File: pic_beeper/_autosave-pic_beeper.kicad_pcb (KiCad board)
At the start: 2 copper layers, 33 x 26.7 mm, 7 parts, among them J1 Conn_01x06, SW1 SW_SPDT, U1 PIC12F752-IP

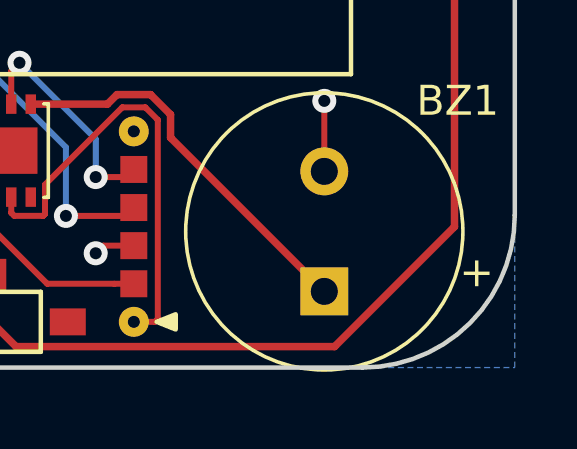
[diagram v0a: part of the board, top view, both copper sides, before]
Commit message: Finish v1.0
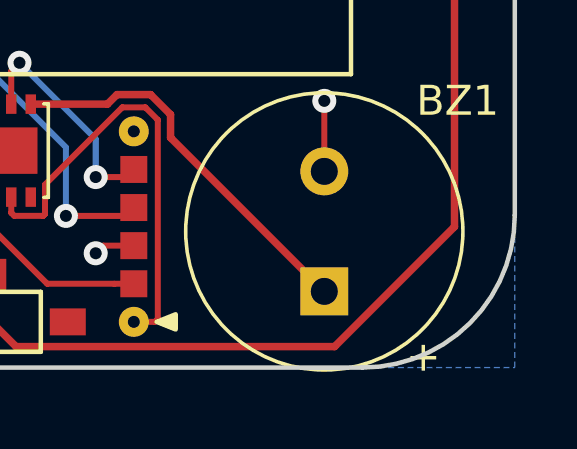
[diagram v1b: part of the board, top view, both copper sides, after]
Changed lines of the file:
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@@
       (outputformat 1)
       (mirror false)
-      (drillshape 1)
+      (drillshape 0)
       (scaleselection 1)
-      (outputdirectory ""))
+      (outputdirectory "plots/"))
   )
   (net 0 "")
@@
       (effects (font (size 1 1) (thickness 0.15)))
     )
-    (fp_text user + (at -5.08 0.635 180) (layer F.SilkS)
+    (fp_text user + (at -3.3 -2.18 180) (layer F.SilkS)
       (effects (font (size 1 1) (thickness 0.15)))
     )
@@
     (pad 6 thru_hole circle (at 2.794 0 90) (size 1 1) (drill 0.4) (layers *.Cu *.Mask)
       (net 8 "Net-(J1-Pad6)"))
-    (pad 5 smd rect (at 1.524 0 90) (size 0.9 0.9) (layers F.Cu F.Paste F.Mask)
+    (pad 5 smd rect (at 1.524 0 90) (size 0.9 0.9) (layers F.Cu F.Mask)
       (net 7 /ICSPCLK))
-    (pad 4 smd rect (at 0.254 0 90) (size 0.9 0.9) (layers F.Cu F.Paste F.Mask)
+    (pad 4 smd rect (at 0.254 0 90) (size 0.9 0.9) (layers F.Cu F.Mask)
       (net 6 /ICSPDAT))
-    (pad 3 smd rect (at -1.016 0 90) (size 0.9 0.9) (layers F.Cu F.Paste F.Mask)
-      (net 2 -BATT))
-    (pad 2 smd rect (at -2.286 0 90) (size 0.9 0.9) (layers F.Cu F.Paste F.Mask)
+    (pad 3 smd rect (at -1.016 0 90) (size 0.9 0.9) (layers F.Cu F.Mask)
+      (net 2 -BATT))
+    (pad 2 smd rect (at -2.286 0 90) (size 0.9 0.9) (layers F.Cu F.Mask)
       (net 4 +BATT))
     (pad 1 thru_hole circle (at -3.556 0 90) (size 1 1) (drill 0.4) (layers *.Cu *.Mask)
@@
       (effects (font (size 1 1) (thickness 0.15)))
     )
+    (fp_circle (center 0 0) (end 3.75 0) (layer F.CrtYd) (width 0.05))
+    (fp_circle (center 0 0) (end 3.5 0) (layer Cmts.User) (width 0.15))
     (fp_text user %R (at 0.3 0) (layer F.Fab)
       (effects (font (size 1 1) (thickness 0.15)))
     )
-    (fp_circle (center 0 0) (end 3.5 0) (layer Cmts.User) (width 0.15))
-    (fp_circle (center 0 0) (end 3.75 0) (layer F.CrtYd) (width 0.05))
+    (pad 1 thru_hole circle (at 1.856155 -1.856155) (size 0.8 0.8) (drill 0.5) (layers *.Cu *.Mask)
+      (net 2 -BATT))
+    (pad 1 thru_hole circle (at 0 -2.625) (size 0.8 0.8) (drill 0.5) (layers *.Cu *.Mask)
+      (net 2 -BATT))
+    (pad 1 thru_hole circle (at -1.856155 -1.856155) (size 0.8 0.8) (drill 0.5) (layers *.Cu *.Mask)
+      (net 2 -BATT))
+    (pad 1 thru_hole circle (at -2.625 0) (size 0.8 0.8) (drill 0.5) (layers *.Cu *.Mask)
+      (net 2 -BATT))
+    (pad 1 thru_hole circle (at -1.856155 1.856155) (size 0.8 0.8) (drill 0.5) (layers *.Cu *.Mask)
+      (net 2 -BATT))
+    (pad 1 thru_hole circle (at 0 2.625) (size 0.8 0.8) (drill 0.5) (layers *.Cu *.Mask)
+      (net 2 -BATT))
+    (pad 1 thru_hole circle (at 1.856155 1.856155) (size 0.8 0.8) (drill 0.5) (layers *.Cu *.Mask)
+      (net 2 -BATT))
+    (pad 1 thru_hole circle (at 2.625 0) (size 0.8 0.8) (drill 0.5) (layers *.Cu *.Mask)
+      (net 2 -BATT))
     (pad 1 thru_hole circle (at 0 0) (size 7 7) (drill 3.5) (layers *.Cu *.Mask)
       (net 2 -BATT))
-    (pad 1 thru_hole circle (at 2.625 0) (size 0.8 0.8) (drill 0.5) (layers *.Cu *.Mask)
-      (net 2 -BATT))
-    (pad 1 thru_hole circle (at 1.856155 1.856155) (size 0.8 0.8) (drill 0.5) (layers *.Cu *.Mask)
-      (net 2 -BATT))
-    (pad 1 thru_hole circle (at 0 2.625) (size 0.8 0.8) (drill 0.5) (layers *.Cu *.Mask)
-      (net 2 -BATT))
-    (pad 1 thru_hole circle (at -1.856155 1.856155) (size 0.8 0.8) (drill 0.5) (layers *.Cu *.Mask)
-      (net 2 -BATT))
-    (pad 1 thru_hole circle (at -2.625 0) (size 0.8 0.8) (drill 0.5) (layers *.Cu *.Mask)
-      (net 2 -BATT))
-    (pad 1 thru_hole circle (at -1.856155 -1.856155) (size 0.8 0.8) (drill 0.5) (layers *.Cu *.Mask)
-      (net 2 -BATT))
-    (pad 1 thru_hole circle (at 0 -2.625) (size 0.8 0.8) (drill 0.5) (layers *.Cu *.Mask)
-      (net 2 -BATT))
-    (pad 1 thru_hole circle (at 1.856155 -1.856155) (size 0.8 0.8) (drill 0.5) (layers *.Cu *.Mask)
-      (net 2 -BATT))
-  )
+  )
